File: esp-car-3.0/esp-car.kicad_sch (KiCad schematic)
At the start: 36 parts, among them J1 Conn_01x07_Socket, J2 Conn_01x07_Socket, U1 ESP32-DEVKIT-V1, U3 L293D

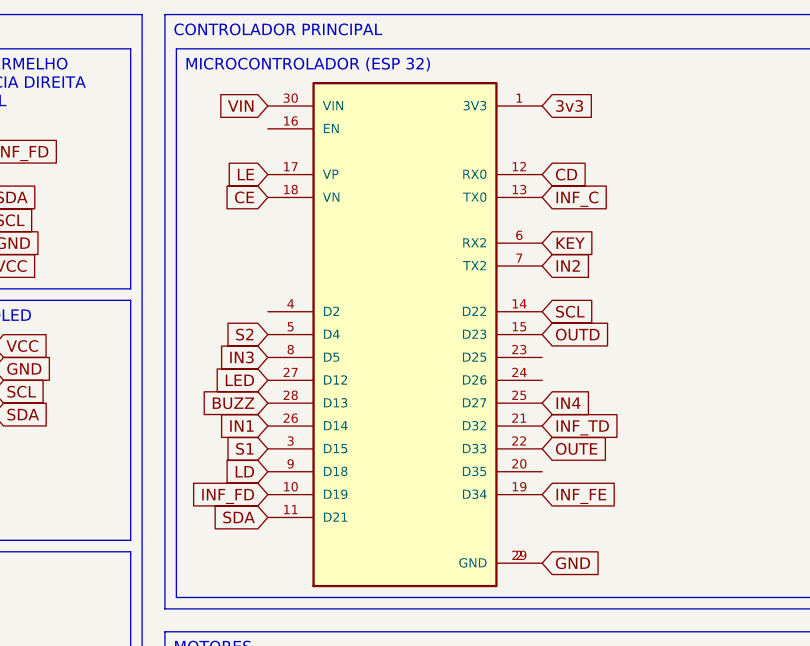
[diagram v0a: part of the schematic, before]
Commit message: finalizada agora
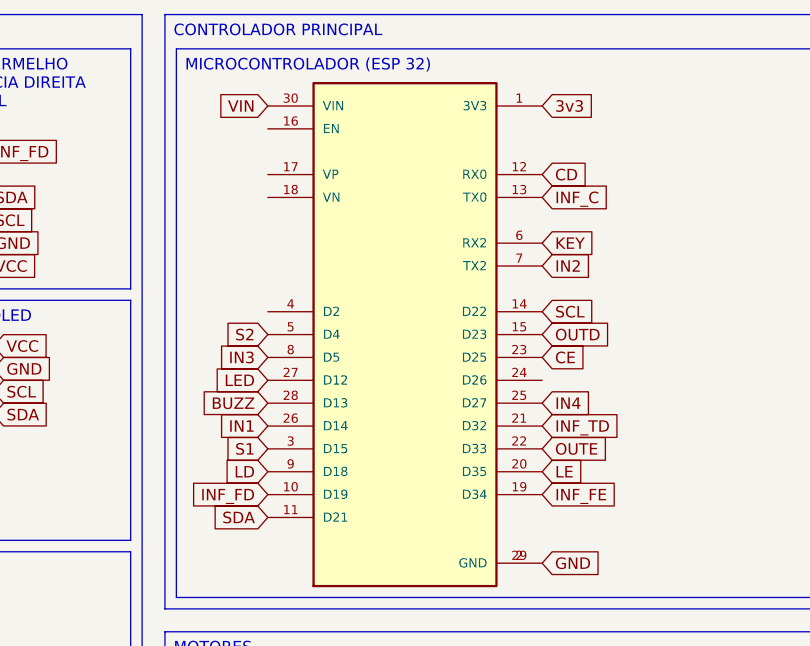
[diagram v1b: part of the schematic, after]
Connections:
- net CE: now also U1.23 (D25); no longer U1.18 (VN)
- net LE: now also U1.20 (D35); no longer U1.17 (VP)
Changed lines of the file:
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@@
 	(global_label "LE"
 		(shape input)
-		(at 96.52 31.75 180)
-		(fields_autoplaced yes)
-		(effects
-			(font
-				(size 1.27 1.27)
-			)
-			(justify right)
-		)
-		(property "Intersheetrefs" "${INTERSHEET_REFS}"
-			(at 91.3577 31.75 0)
-			(effects
-				(font
-					(size 1.27 1.27)
-				)
-				(justify right)
+		(at 127 64.77 0)
+		(fields_autoplaced yes)
+		(effects
+			(font
+				(size 1.27 1.27)
+			)
+			(justify left)
+		)
+		(property "Intersheetrefs" "${INTERSHEET_REFS}"
+			(at 132.1623 64.77 0)
+			(effects
+				(font
+					(size 1.27 1.27)
+				)
+				(justify left)
 				(hide yes)
 			)
@@
 	(global_label "CE"
 		(shape input)
-		(at 96.52 34.29 180)
-		(fields_autoplaced yes)
-		(effects
-			(font
-				(size 1.27 1.27)
-			)
-			(justify right)
-		)
-		(property "Intersheetrefs" "${INTERSHEET_REFS}"
-			(at 91.1158 34.29 0)
-			(effects
-				(font
-					(size 1.27 1.27)
-				)
-				(justify right)
-				(hide yes)
-			)
+		(at 127 52.07 0)
+		(fields_autoplaced yes)
+		(effects
+			(font
+				(size 1.27 1.27)
+			)
+			(justify left)
+		)
+		(property "Intersheetrefs" "${INTERSHEET_REFS}"
+			(at 132.4042 52.07 0)
+			(effects
+				(font
+					(size 1.27 1.27)
+				)
+				(justify left)
+				(hide yes)
+			)
